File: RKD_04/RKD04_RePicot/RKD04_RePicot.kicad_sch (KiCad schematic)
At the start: 5 parts, among them J1 Conn_01x08, J2 Conn_01x24, J3 Qwiic_RA, U1 Pico

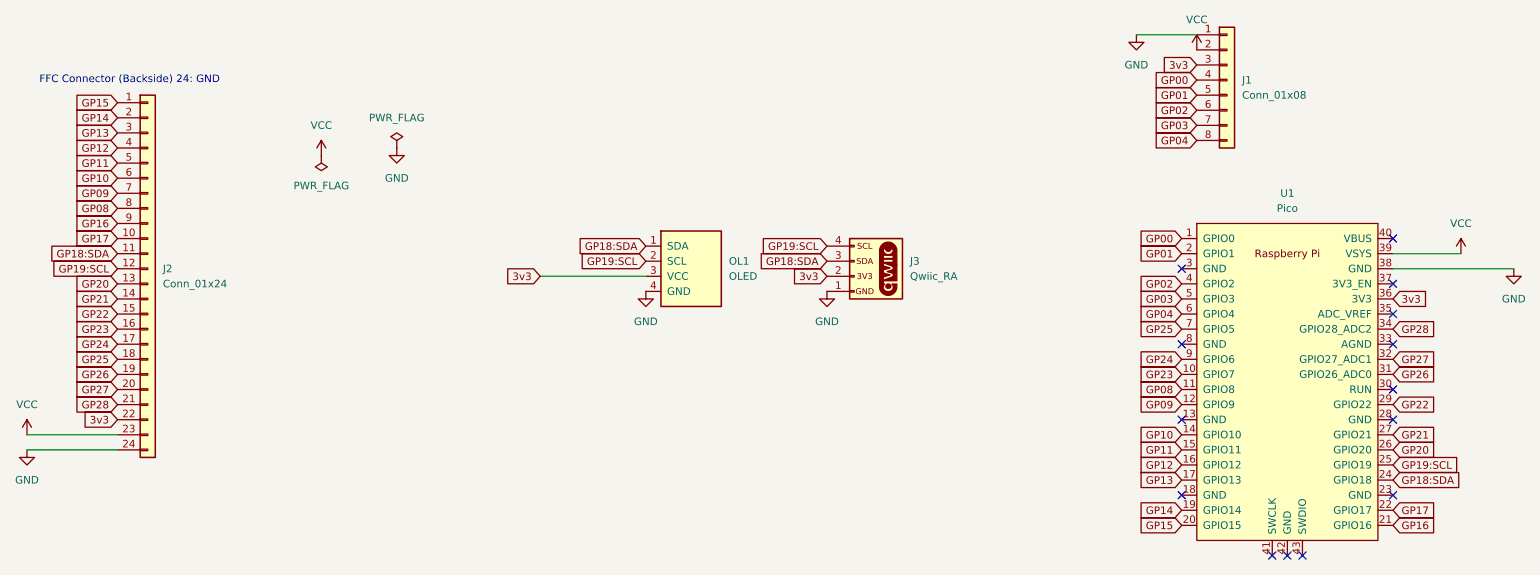
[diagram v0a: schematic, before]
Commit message: RePicot 更新
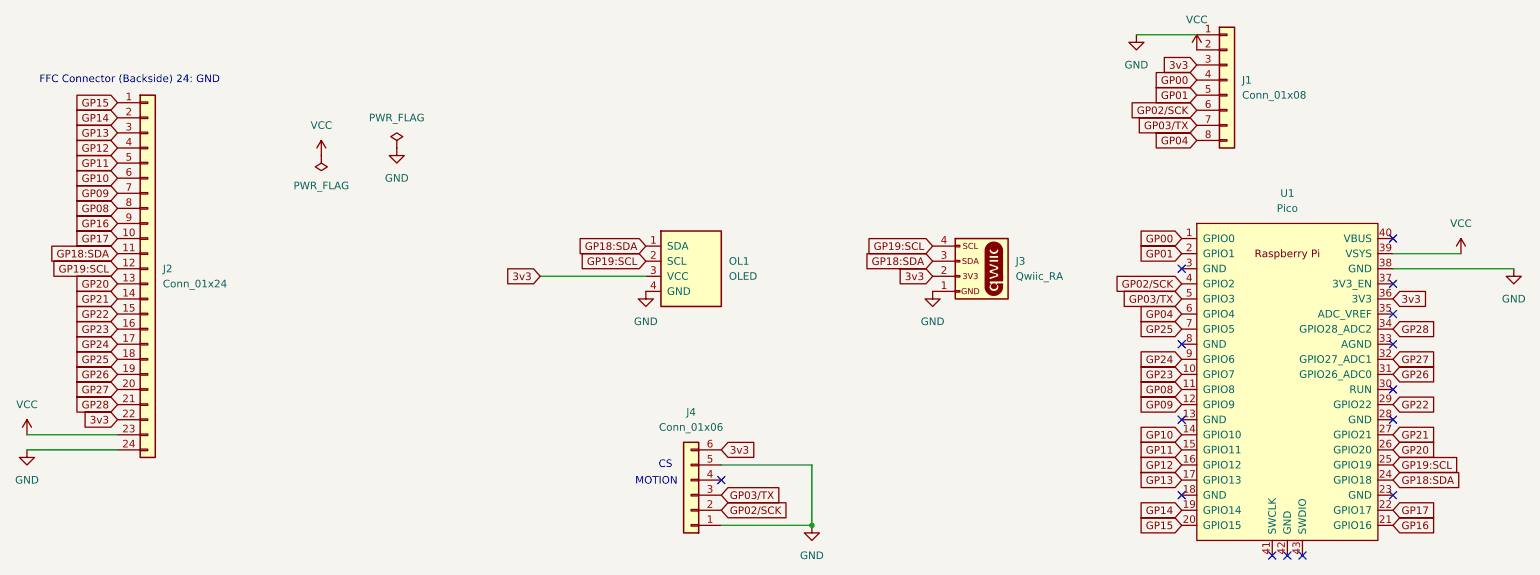
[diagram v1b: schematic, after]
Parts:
- added J4: Conn_01x06, Connector_FFC-FPC:Hirose_FH12-6S-0.5SH_1x06-1MP_P0.50mm_Horizontal, symbol Connector_Generic:Conn_01x06
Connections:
- net 3v3: now also J4.6 (Pin_6)
- net GND: now also J4.1 (Pin_1), J4.5 (Pin_5)
- net GP02 renamed GP02/SCK
- net GP02/SCK: now also J4.2 (Pin_2)
- net GP03 renamed GP03/TX
- net GP03/TX: now also J4.3 (Pin_3)
- no-connect marks 14 -> 15
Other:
- note added: "CS"
- note added: "MOTION"
- moved on the sheet: J3
